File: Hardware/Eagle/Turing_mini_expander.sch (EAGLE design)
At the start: 20 parts, among them U1 TL072_

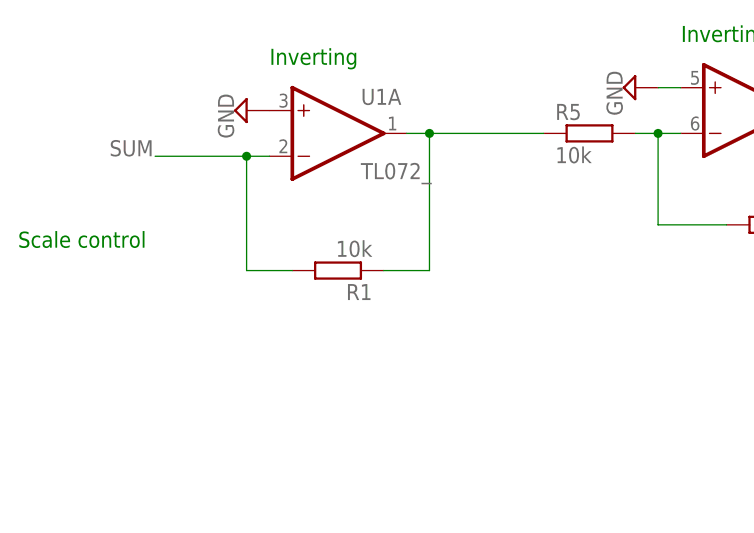
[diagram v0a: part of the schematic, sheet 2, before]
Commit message: Merge remote-tracking branch 'origin/master'
Conflicts:
	Hardware/Eagle/Turing_mini_expander.brd
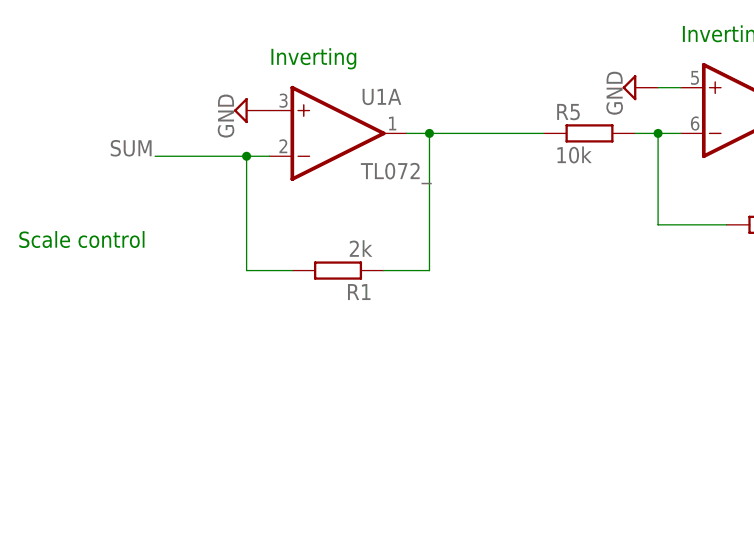
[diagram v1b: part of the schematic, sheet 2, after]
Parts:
- R1: value 10k -> 2k
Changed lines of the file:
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@@
 <part name="VR5" library="MusicThingModular" deviceset="9MM_SNAP-IN_POT_CHASSIS" device=""/>
 <part name="VR6" library="MusicThingModular" deviceset="9MM_SNAP-IN_POT_CHASSIS" device=""/>
-<part name="R1" library="MusicThingModular" deviceset="RESISTOR" device="7MM" value="10k"/>
+<part name="R1" library="MusicThingModular" deviceset="RESISTOR" device="7MM" value="2k"/>
 <part name="R2" library="MusicThingModular" deviceset="RESISTOR" device="7MM" value="10k"/>
 <part name="R3" library="MusicThingModular" deviceset="RESISTOR" device="7MM" value="10k"/>

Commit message: Revert "Merge remote-tracking branch 'origin/master'"
This reverts commit c677e9c759e717a54841b66673ad6128330ede4f.
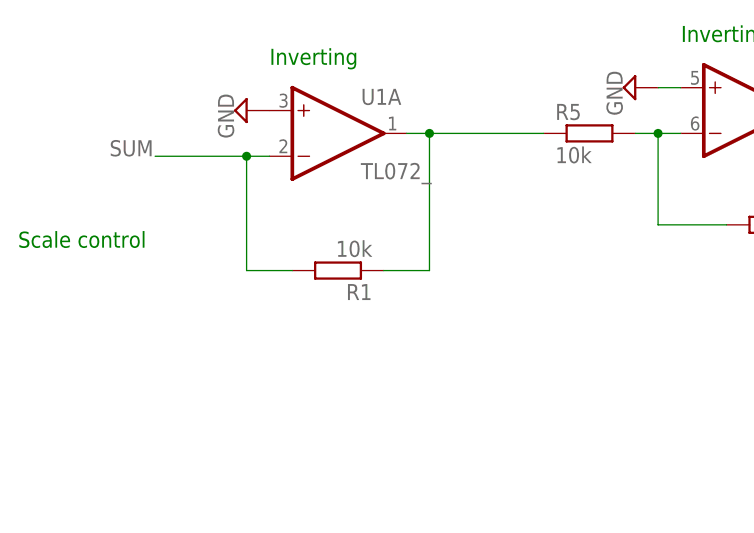
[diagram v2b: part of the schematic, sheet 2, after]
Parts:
- R1: value 2k -> 10k
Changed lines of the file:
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@@
 <part name="VR5" library="MusicThingModular" deviceset="9MM_SNAP-IN_POT_CHASSIS" device=""/>
 <part name="VR6" library="MusicThingModular" deviceset="9MM_SNAP-IN_POT_CHASSIS" device=""/>
-<part name="R1" library="MusicThingModular" deviceset="RESISTOR" device="7MM" value="2k"/>
+<part name="R1" library="MusicThingModular" deviceset="RESISTOR" device="7MM" value="10k"/>
 <part name="R2" library="MusicThingModular" deviceset="RESISTOR" device="7MM" value="10k"/>
 <part name="R3" library="MusicThingModular" deviceset="RESISTOR" device="7MM" value="10k"/>
